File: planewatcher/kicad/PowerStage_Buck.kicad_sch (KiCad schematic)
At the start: 19 parts, among them U12 LT8640IUDCF-1#PBF

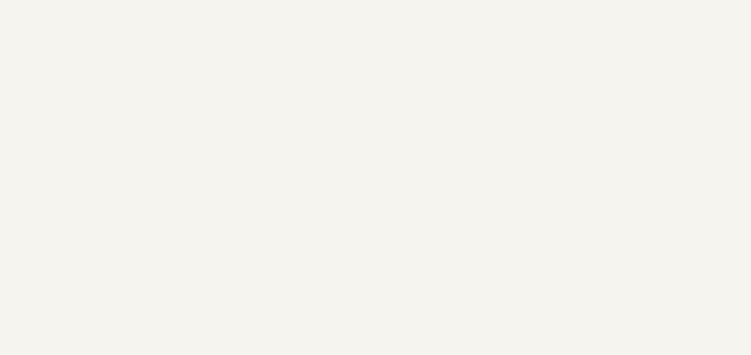
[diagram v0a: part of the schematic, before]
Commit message: updates before fab
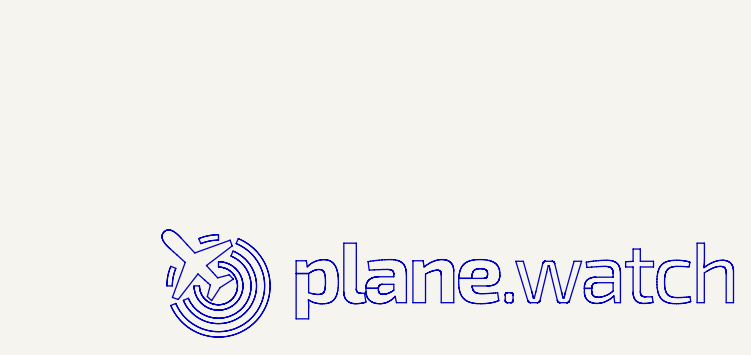
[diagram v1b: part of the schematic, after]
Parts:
- C59, C60: Purpose (none) -> Input ceramic capacitor for the LT8640 buck regulator.; Suggested Part (none) -> Murata GRM31CR71E475KA88L
- C61, C62: Purpose (none) -> Local 1µF VIN bypass capacitor for the LT8640 buck regulato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; Suggested Part (none) -> Murata GRM188R61C105KA93D
- C63: Purpose (none) -> LT8640 BST-to-SW bootstrap capacitor for the high-side swit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; Suggested Part (none) -> Murata GRM155R71H104KE14D
- C64: Purpose (none) -> Soft-start or regulator control bypass capacitor in the LT8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; Suggested Part (none) -> Murata GRM155R71H103KA88D
- C65: Purpose (none) -> Feed-forward/compensation capacitor across the LT8640 feedb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; Suggested Part (none) -> Murata GRM1555C1H4R7CA01D
- C66: Purpose (none) -> LT8640 output bulk capacitor for FPGA rail ripple and load 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; Suggested Part (none) -> KEMET C1210C476M4PACTU
- C67: Purpose (none) -> Regulator auxiliary/input bypass capacitor in the LT8640 bu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; Suggested Part (none) -> Murata GRM155R61C105KA12D
- JP1: Purpose (none) -> Allows the FPGA power rail to be linked or isolated during 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; Suggested Part (none) -> Samtec TSW-102-07-L-S
- L10: Purpose (none) -> LT8640 buck switching inductor for the FPGA 5V supply.; Suggested Part (none) -> Coilcraft XAL5030-472ME
- L9: Purpose (none) -> Filters high-frequency switching noise on the LT8640 regula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; Suggested Part (none) -> Murata BLM21PG600SN1D
- R32: Purpose (none) -> LT8640 power-good pull-up or regulator status bias resistor.; Suggested Part (none) -> Yageo RC0402FR-0747KL
- R33: Purpose (none) -> Top feedback resistor setting the LT8640 FPGA 5V output vol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; Suggested Part (none) -> Yageo RC0402FR-071ML
- R34: Purpose (none) -> Bottom/trim feedback resistor setting the LT8640 output vol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; Suggested Part (none) -> Yageo RC0402FR-07243KL
- R35: Purpose (none) -> LT8640 RT resistor setting the FPGA buck switching frequenc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; Suggested Part (none) -> Yageo RC0402FR-0760K4L
- TP18: Purpose (none) -> Provides oscilloscope/DMM probe access to VOUT.; Suggested Part (none) -> No fitted part (PCB pad only); now left out of the parts list
- TP19: Purpose (none) -> Provides oscilloscope/DMM probe access to PG.; Suggested Part (none) -> No fitted part (PCB pad only); now left out of the parts list
- U12: Purpose (none) -> Generates the FPGA 5V rail from the protected input supply.; Suggested Part (none) -> Analog Devices LT8640IUDCF-1#PBF
